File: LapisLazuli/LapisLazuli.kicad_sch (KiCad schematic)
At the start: 0 parts

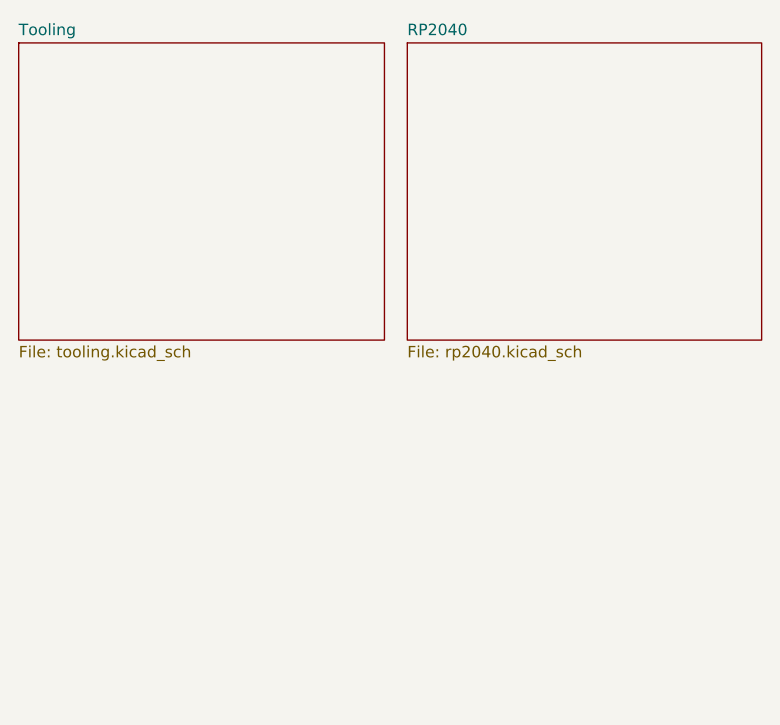
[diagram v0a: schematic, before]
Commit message: Zaid Schematic Review
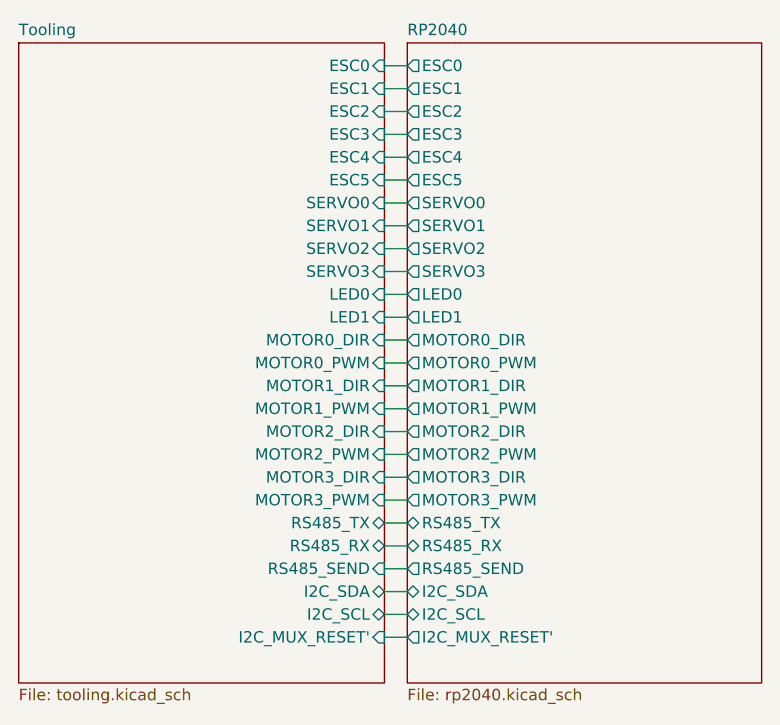
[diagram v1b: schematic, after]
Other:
- sheet RP2040 ports: added ESC0, ESC1, ESC2, ESC3, ESC4, ESC5, I2C_MUX_RESET', I2C_SCL, I2C_SDA, LED0, LED1, MOTOR0_DIR, MOTOR0_PWM, MOTOR1_DIR, MOTOR1_PWM, MOTOR2_DIR, MOTOR2_PWM, MOTOR3_DIR, MOTOR3_PWM, RS485_RX, RS485_SEND, RS485_TX, SERVO0, SERVO1, SERVO2, SERVO3; removed none
- sheet Tooling ports: added ESC0, ESC1, ESC2, ESC3, ESC4, ESC5, I2C_MUX_RESET', I2C_SCL, I2C_SDA, LED0, LED1, MOTOR0_DIR, MOTOR0_PWM, MOTOR1_DIR, MOTOR1_PWM, MOTOR2_DIR, MOTOR2_PWM, MOTOR3_DIR, MOTOR3_PWM, RS485_RX, RS485_SEND, RS485_TX, SERVO0, SERVO1, SERVO2, SERVO3; removed none
